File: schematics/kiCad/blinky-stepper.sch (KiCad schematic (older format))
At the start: 10 parts, among them J1 PJ-102A, U1 Teensy-LC, U2 HC06

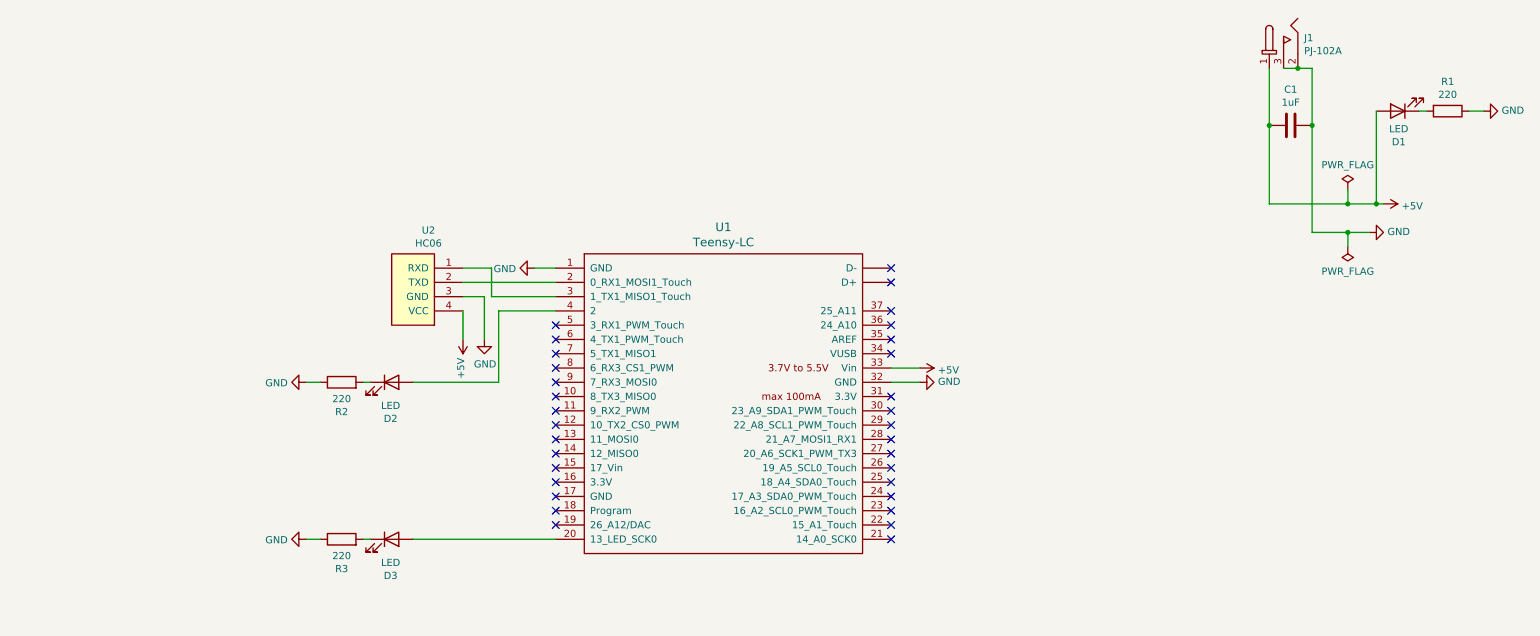
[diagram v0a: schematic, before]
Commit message: pcb finished
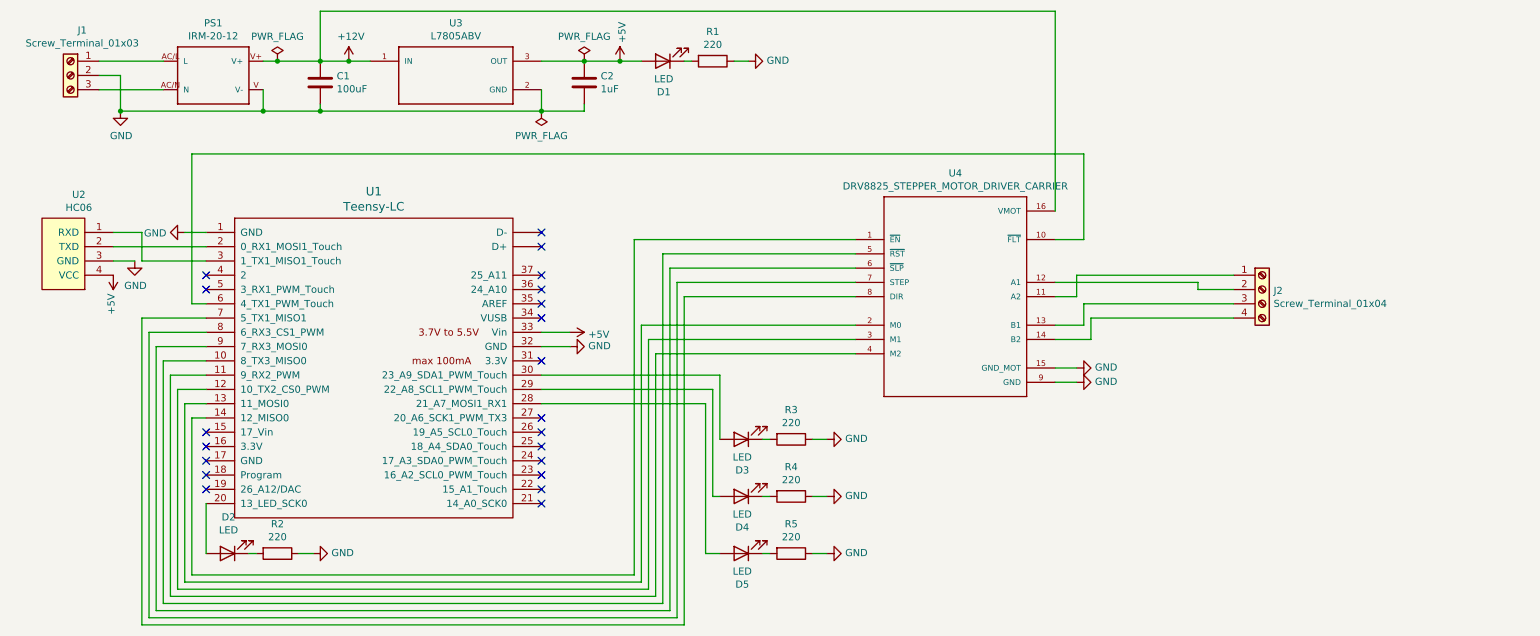
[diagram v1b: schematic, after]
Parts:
- removed D2: LED, LED_THT:LED_D5.0mm, symbol Device:LED
- removed J1: PJ-102A, dmcginnis427:DC21Jack, symbol blinky-lite-basic-rescue:PJ-102A-dk_Barrel-Power-Connectors
- removed R2: 220, Resistor_SMD:R_1206_3216Metric_Pad1.42x1.75mm_HandSolder, symbol Device:R
- added C2: 1uF, Capacitor_SMD:C_1206_3216Metric_Pad1.42x1.75mm_HandSolder, symbol Device:C
- added D3, D4, D5: LED, LED_THT:LED_D5.0mm, symbol Device:LED
- added J1: Screw_Terminal_01x03, TerminalBlock:TerminalBlock_bornier-3_P5.08mm, symbol Connector:Screw_Terminal_01x03
- added J2: Screw_Terminal_01x04, TerminalBlock:TerminalBlock_bornier-4_P5.08mm, symbol Connector:Screw_Terminal_01x04
- added PS1: IRM-20-12, IRM-20-12:IRM-20-12, symbol IRM-20-12:IRM-20-12
- added R3, R4, R5: 220, Resistor_SMD:R_1206_3216Metric_Pad1.42x1.75mm_HandSolder, symbol Device:R
- added U3: L7805ABV, L7805ABV:TO254P460X1020X1945-3P, symbol L7805ABV:L7805ABV
- added U4: DRV8825_STEPPER_MOTOR_DRIVER_CARRIER, DRV8825:IC_DRV8825_STEPPER_MOTOR_DRIVER_CARRIER, symbol DRV8825:DRV8825_STEPPER_MOTOR_DRIVER_CARRIER
- C1: value 1uF -> 100uF; footprint Capacitor_SMD:C_1206_3216Metric_Pad1.42x1.75mm_HandSolder -> Capacitor_THT:CP_Radial_D10.0mm_P5.00mm
- U2: footprint dmcginnis427:HC06 -> dmcginnis427Footprints:HC06
- renumbered D3 to D2, R3 to R2
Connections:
- net +5V: now also C2.1, U3.3 (OUT); no longer C1.2
- net GND: now also C1.2, C2.2, J1.2 (Pin_2), PS1.V (V-), R3.1, R4.1, R5.1, U3.2 (GND), U4.15 (GND_MOT), U4.9 (GND); no longer C1.1
- net at U1.10 (8_TX3_MISO0): now also U4.5 (~RST~)
- net at U1.11 (9_RX2_PWM): now also U4.4 (M2)
- net at U1.12 (10_TX2_CS0_PWM): now also U4.3 (M1)
- net at U1.13 (11_MOSI0): now also U4.2 (M0)
- net at U1.14 (12_MISO0): now also U4.1 (~EN~)
- net at U1.28 (21_A7_MOSI1_RX1): now also D5.2 (A)
- net at U1.29 (22_A8_SCL1_PWM_Touch): now also D4.2 (A)
- net at U1.30 (23_A9_SDA1_PWM_Touch): now also D3.2 (A)
- net at U1.6 (4_TX1_PWM_Touch): now also U4.10 (~FLT~)
- net at U1.7 (5_TX1_MISO1): now also U4.8 (DIR)
- net at U1.8 (6_RX3_CS1_PWM): now also U4.7 (STEP)
- net at U1.9 (7_RX3_MOSI0): now also U4.6 (~SLP~)
- new net: J1.1 (Pin_1), PS1.AC/L (L)
- new net: J1.3 (Pin_3), PS1.AC/N (N)
- new net: D3.1 (K), R3.2
- new net: D4.1 (K), R4.2
- new net: D5.1 (K), R5.2
- new net: J2.1 (Pin_1), U4.11 (A2)
- new net: J2.2 (Pin_2), U4.12 (A1)
- new net: J2.3 (Pin_3), U4.13 (B1)
- new net: J2.4 (Pin_4), U4.14 (B2)
- new net +12V: C1.1, PS1.V+, U3.1 (IN), U4.16 (VMOT)
- no-connect marks 32 -> 21
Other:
- moved on the sheet: D1, D2, R1, R2, U1, U2
